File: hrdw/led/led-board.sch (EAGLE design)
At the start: 3 parts, among them U1 MAX4232AKA+

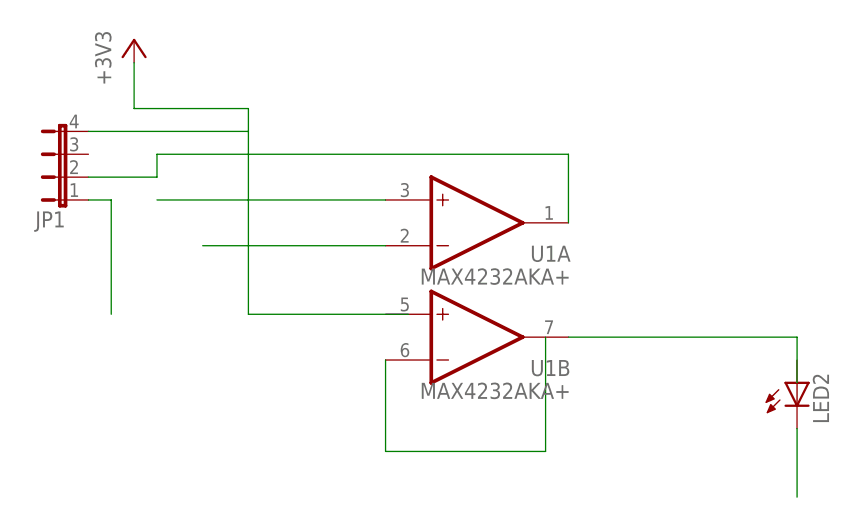
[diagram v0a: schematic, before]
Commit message: [sleepwaler] code cleanup.
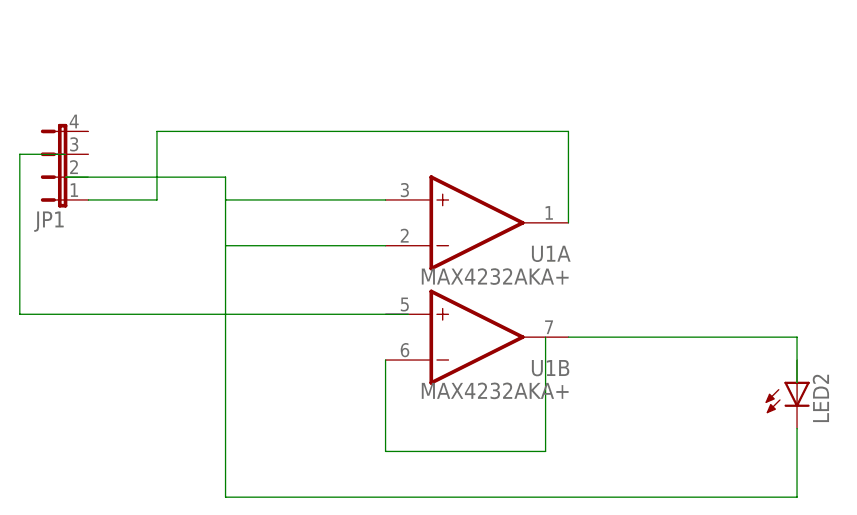
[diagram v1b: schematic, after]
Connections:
- removed net +3V3: JP1.4
- removed net N$11: U1A.+IN
- removed net N$3: U1A.-IN
- removed net N$5: JP1.2, U1A.OUT
- net N$2: now also JP1.1, U1A.OUT; no longer LED2.C
- net N$8: now also LED2.C, U1A.+IN, U1A.-IN; no longer JP1.1
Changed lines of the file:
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@@
 <part name="LED2" library="led" deviceset="LED" device="CHIPLED-0603-TTW"/>
 <part name="U1" library="_MAX4230_MAX4231_MAX4232_MAX4234" deviceset="MAX4232*" device="AKA+"/>
-<part name="+3V1" library="supply1" deviceset="+3V3" device=""/>
 <part name="JP1" library="jumper" deviceset="JP4E" device=""/>
 </parts>
@@
 <instance part="U1" gate="A" x="38.1" y="66.04"/>
 <instance part="U1" gate="B" x="38.1" y="53.34"/>
-<instance part="+3V1" gate="G$1" x="0" y="86.36"/>
 <instance part="JP1" gate="G$1" x="-7.62" y="71.12" rot="R90"/>
 </instances>
@@
 </segment>
 </net>
-<net name="+3V3" class="0">
-<segment>
-<pinref part="+3V1" gate="G$1" pin="+3V3"/>
-<wire x1="0" y1="83.82" x2="0" y2="78.74" width="0.1524" layer="91"/>
-<wire x1="0" y1="78.74" x2="12.7" y2="78.74" width="0.1524" layer="91"/>
-<wire x1="12.7" y1="78.74" x2="12.7" y2="76.2" width="0.1524" layer="91"/>
-<wire x1="12.7" y1="76.2" x2="12.7" y2="55.88" width="0.1524" layer="91"/>
-<wire x1="12.7" y1="55.88" x2="30.48" y2="55.88" width="0.1524" layer="91"/>
-<pinref part="JP1" gate="G$1" pin="4"/>
-<wire x1="-5.08" y1="76.2" x2="12.7" y2="76.2" width="0.1524" layer="91"/>
-</segment>
-</net>
 <net name="N$4" class="0">
 <segment>
@@
 </segment>
 </net>
-<net name="N$5" class="0">
-<segment>
-<pinref part="JP1" gate="G$1" pin="2"/>
-<wire x1="-5.08" y1="71.12" x2="2.54" y2="71.12" width="0.1524" layer="91"/>
-<wire x1="2.54" y1="71.12" x2="2.54" y2="73.66" width="0.1524" layer="91"/>
-<wire x1="2.54" y1="73.66" x2="48.26" y2="73.66" width="0.1524" layer="91"/>
-<pinref part="U1" gate="A" pin="OUT"/>
-<wire x1="48.26" y1="73.66" x2="48.26" y2="66.04" width="0.1524" layer="91"/>
-</segment>
-</net>
-<net name="N$11" class="0">
-<segment>
-<pinref part="U1" gate="A" pin="+IN"/>
-<wire x1="27.94" y1="68.58" x2="2.54" y2="68.58" width="0.1524" layer="91"/>
-</segment>
-</net>
 <net name="N$2" class="0">
 <segment>
-<pinref part="LED2" gate="G$1" pin="C"/>
-<wire x1="73.66" y1="43.18" x2="73.66" y2="35.56" width="0.1524" layer="91"/>
-</segment>
-</net>
-<net name="N$3" class="0">
-<segment>
-<pinref part="U1" gate="A" pin="-IN"/>
-<wire x1="27.94" y1="63.5" x2="7.62" y2="63.5" width="0.1524" layer="91"/>
+<wire x1="2.54" y1="76.2" x2="48.26" y2="76.2" width="0.1524" layer="91"/>
+<pinref part="U1" gate="A" pin="OUT"/>
+<wire x1="48.26" y1="76.2" x2="48.26" y2="66.04" width="0.1524" layer="91"/>
+<wire x1="2.54" y1="76.2" x2="2.54" y2="68.58" width="0.1524" layer="91"/>
+<pinref part="JP1" gate="G$1" pin="1"/>
+<wire x1="2.54" y1="68.58" x2="-5.08" y2="68.58" width="0.1524" layer="91"/>
 </segment>
 </net>
 <net name="N$8" class="0">
 <segment>
-<pinref part="JP1" gate="G$1" pin="1"/>
-<wire x1="-5.08" y1="68.58" x2="-2.54" y2="68.58" width="0.1524" layer="91"/>
-<wire x1="-2.54" y1="68.58" x2="-2.54" y2="55.88" width="0.1524" layer="91"/>
+<pinref part="U1" gate="A" pin="+IN"/>
+<wire x1="27.94" y1="68.58" x2="10.16" y2="68.58" width="0.1524" layer="91"/>
+<pinref part="U1" gate="A" pin="-IN"/>
+<wire x1="27.94" y1="63.5" x2="10.16" y2="63.5" width="0.1524" layer="91"/>
+<wire x1="10.16" y1="68.58" x2="10.16" y2="63.5" width="0.1524" layer="91"/>
+<wire x1="10.16" y1="63.5" x2="10.16" y2="35.56" width="0.1524" layer="91"/>
+<pinref part="LED2" gate="G$1" pin="C"/>
+<wire x1="73.66" y1="43.18" x2="73.66" y2="35.56" width="0.1524" layer="91"/>
+<wire x1="10.16" y1="35.56" x2="73.66" y2="35.56" width="0.1524" layer="91"/>
+<wire x1="10.16" y1="68.58" x2="10.16" y2="71.12" width="0.1524" layer="91"/>
+<wire x1="10.16" y1="71.12" x2="-7.62" y2="71.12" width="0.1524" layer="91"/>
 </segment>
 </net>
+<net name="N$6" class="0">
+<segment>
+<wire x1="-12.7" y1="55.88" x2="30.48" y2="55.88" width="0.1524" layer="91"/>
+<wire x1="-12.7" y1="55.88" x2="-12.7" y2="73.66" width="0.1524" layer="91"/>
+<wire x1="-12.7" y1="73.66" x2="-7.62" y2="73.66" width="0.1524" layer="91"/>
+</segment>
+</net>
